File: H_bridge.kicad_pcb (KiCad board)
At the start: 2 copper layers, 32 x 21 mm, 24 parts, among them J1 Conn_01x04_Socket, J2 Conn_01x04_Socket, J3 Conn_01x04_Socket, J4 Conn_01x04_Socket, J5 Conn_01x04_Socket, J6 Conn_01x04_Socket, J7 Conn_01x04_Socket, J8 Conn_01x04_Socket, U1 VNH7040AYTR

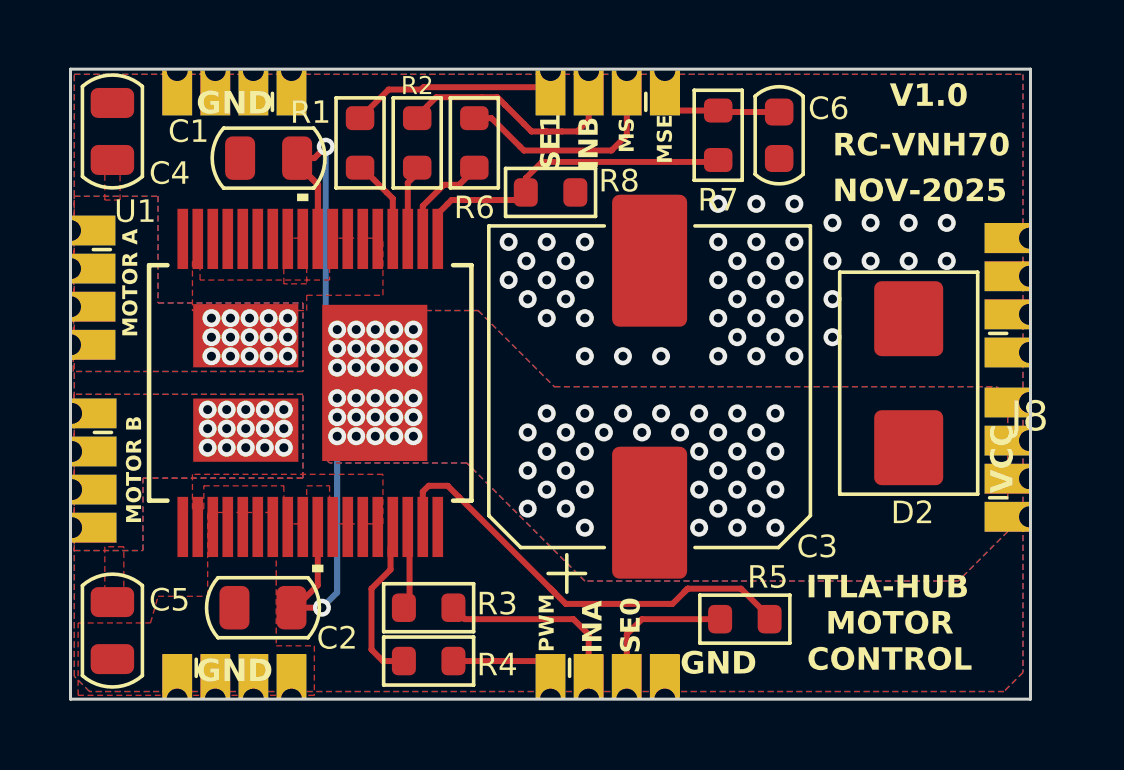
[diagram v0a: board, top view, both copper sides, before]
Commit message: Version 1 enviada a fabricacion
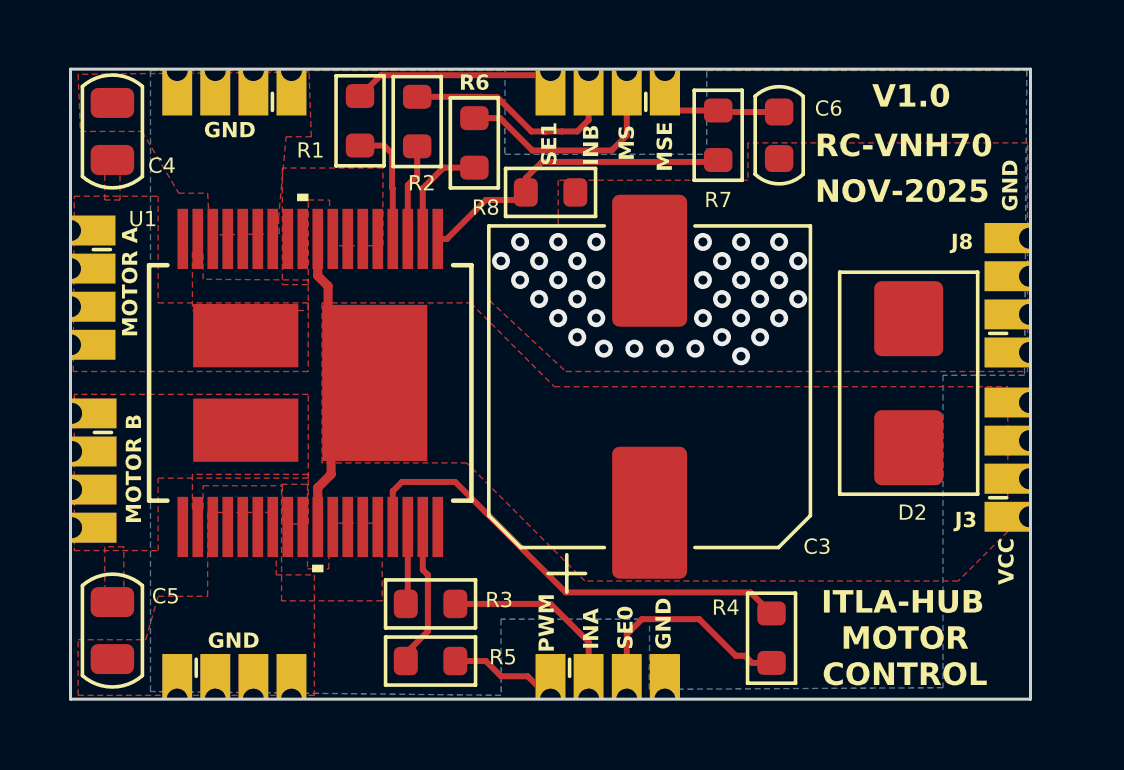
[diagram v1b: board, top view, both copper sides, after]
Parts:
- removed C1, C2: C_0805, Capacitor_SMD_AKL:C_0805_2012Metric
- C4, C5: value C_0805 -> 100NF
- R1: value 1k -> 1K
- R2, R3, R4, R5, R6: value R_0603 -> 1K
- R7: value 10k -> 10K
- R8: value 1k -> 1.5K
- moved R4 11.5 mm to (135.6, 83.7), turned to 90 degrees
- moved R5 10.6 mm to (124.3, 84.5), turned to 180 degrees
- moved R1 0.74 mm to (121.9, 66.5)
- moved R2 0.71 mm to (123.8, 66.5)
- moved R3 0.14 mm to (124.3, 82.6)
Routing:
- net Net-(U1-Sel0): track 4.93 -> 15.8 mm
- net Net-(U1-PWM): track 15.3 -> 4.95 mm
- net VCC: track 22.6 -> 12.9 mm, vias 68 -> 0
- net /sel0: track 2.98 -> 7.80 mm
- net Net-(U1-Sel1): track 2.84 -> 4.03 mm
- net /in_a: track 6.02 -> 6.94 mm
- net /pwm: track 4.34 -> 5.22 mm
- net Net-(U1-Input_B): track 2.49 -> 3.22 mm
- net GND: vias 46 -> 36
- net /motor_b: vias 15 -> 0
- net /motor_a: vias 15 -> 0
- removed copper zone on B.Cu, net /motor_a
- removed copper zone on B.Cu, net /motor_b
- removed copper zone on B.Cu, net VCC
